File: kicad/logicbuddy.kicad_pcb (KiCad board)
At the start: 2 copper layers, 130 x 100 mm, 33 parts, among them J1 USB_C_2PIN, Q1 NPN, Q2 NPN, Q3 NPN, Q4 NPN, Q5 NPN, Q6 NPN, Q7 NPN, SW1 SW_SPST, SW2 SW_SPST, SW3 SW_SPST, SW4 SW_SPST, SW5 SW_SPST, SW6 SW_SPST, SW7 SW_SPST, SW8 SW_DIP_x01

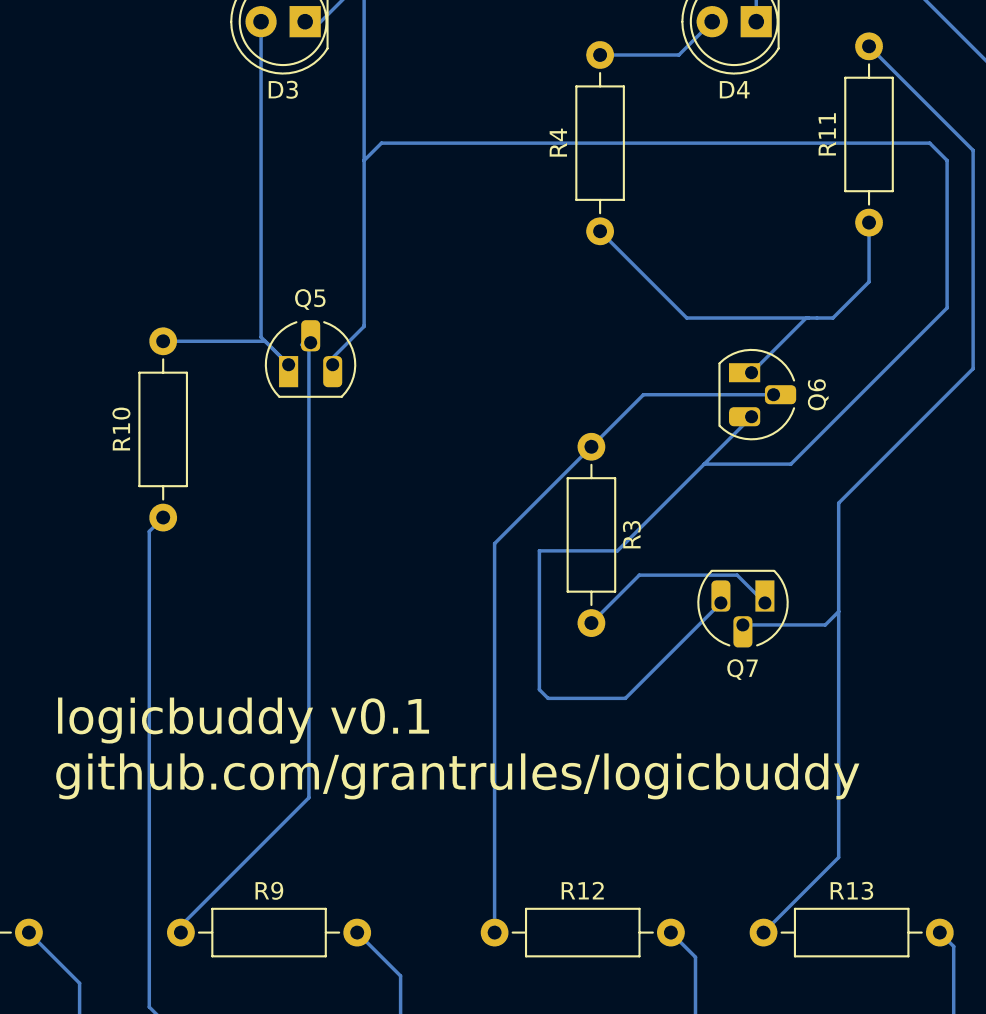
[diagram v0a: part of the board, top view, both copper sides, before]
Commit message: Reapply "updated labels and fixed footprints"
This reverts commit 2a946a7896d612220efc5a586cb72ca7f3163489.
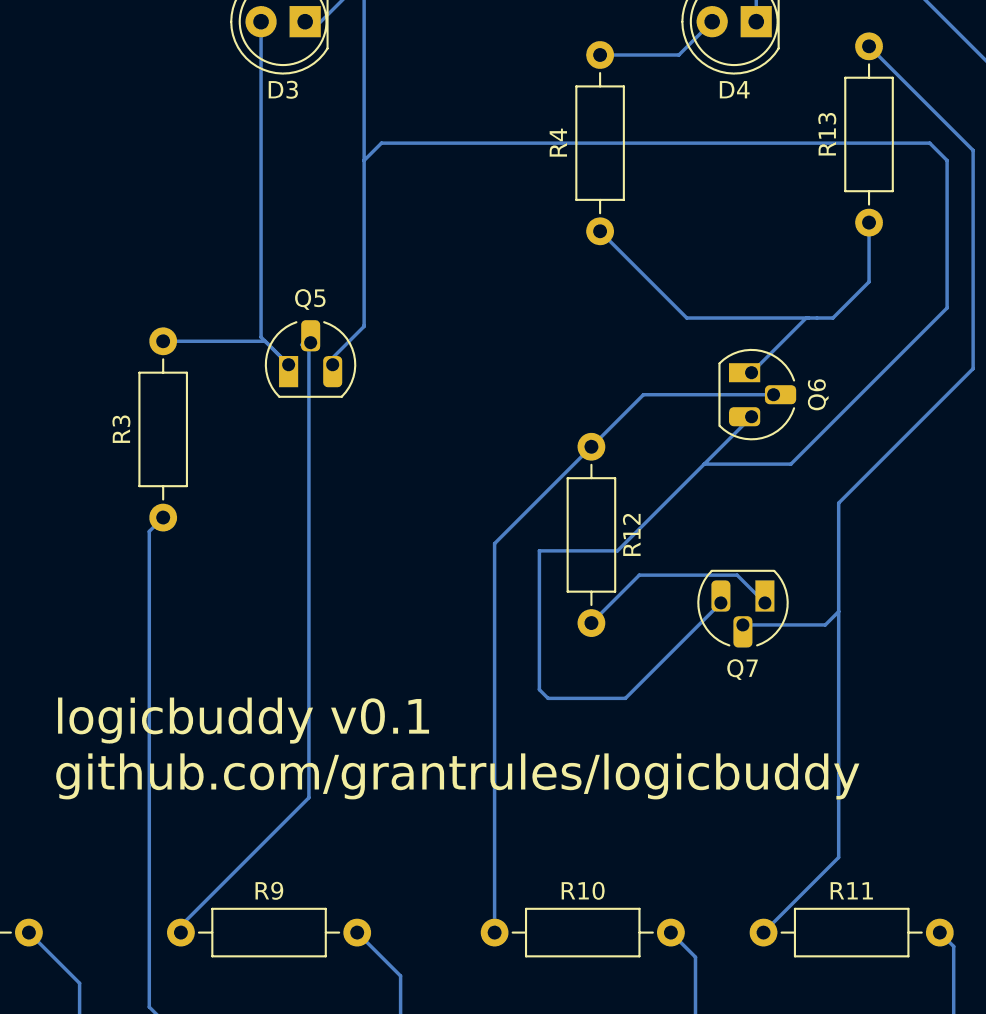
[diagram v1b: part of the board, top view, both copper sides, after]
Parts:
- renumbered R12 to R10, R13 to R11, R3 to R12, R11 to R13, R10 to R3

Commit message: Revert "updated labels and fixed footprints"
This reverts commit cc8675b157493e85bb3edc9923989f4c8e1865eb.
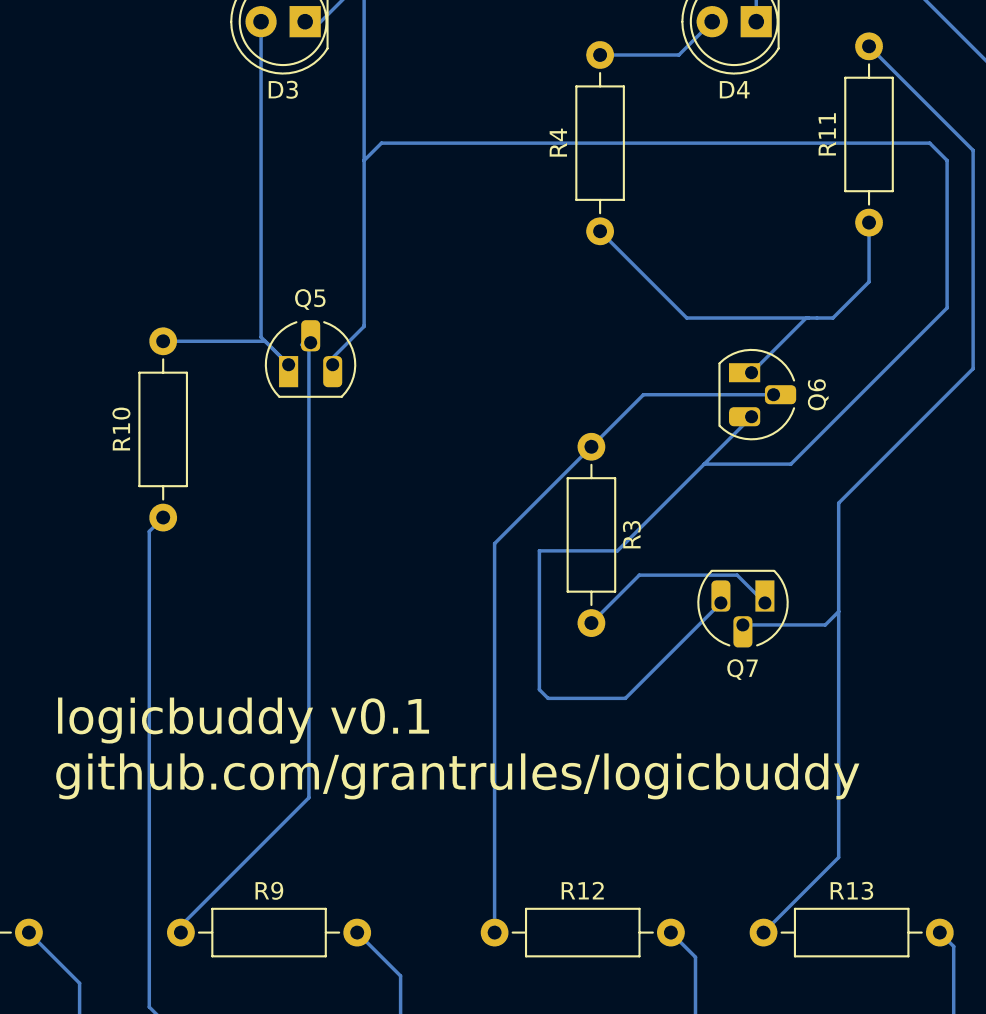
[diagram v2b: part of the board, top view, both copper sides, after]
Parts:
- renumbered R3 to R10, R13 to R11, R10 to R12, R11 to R13, R12 to R3
